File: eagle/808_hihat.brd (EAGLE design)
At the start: 100 x 80 mm, 103 parts, among them IC1 TL072P, IC3 TL071P, Q1 2N3904, Q10 2N3904, Q11 2N3904, Q12 2N3904, Q13 2N3906, Q14 2N3906, Q2 2N3904, Q3 2N3904, Q4 2N3904, Q5 2N3904, Q6 2N3904, Q7 2N3904, Q8 2N3904, Q9 2N3904

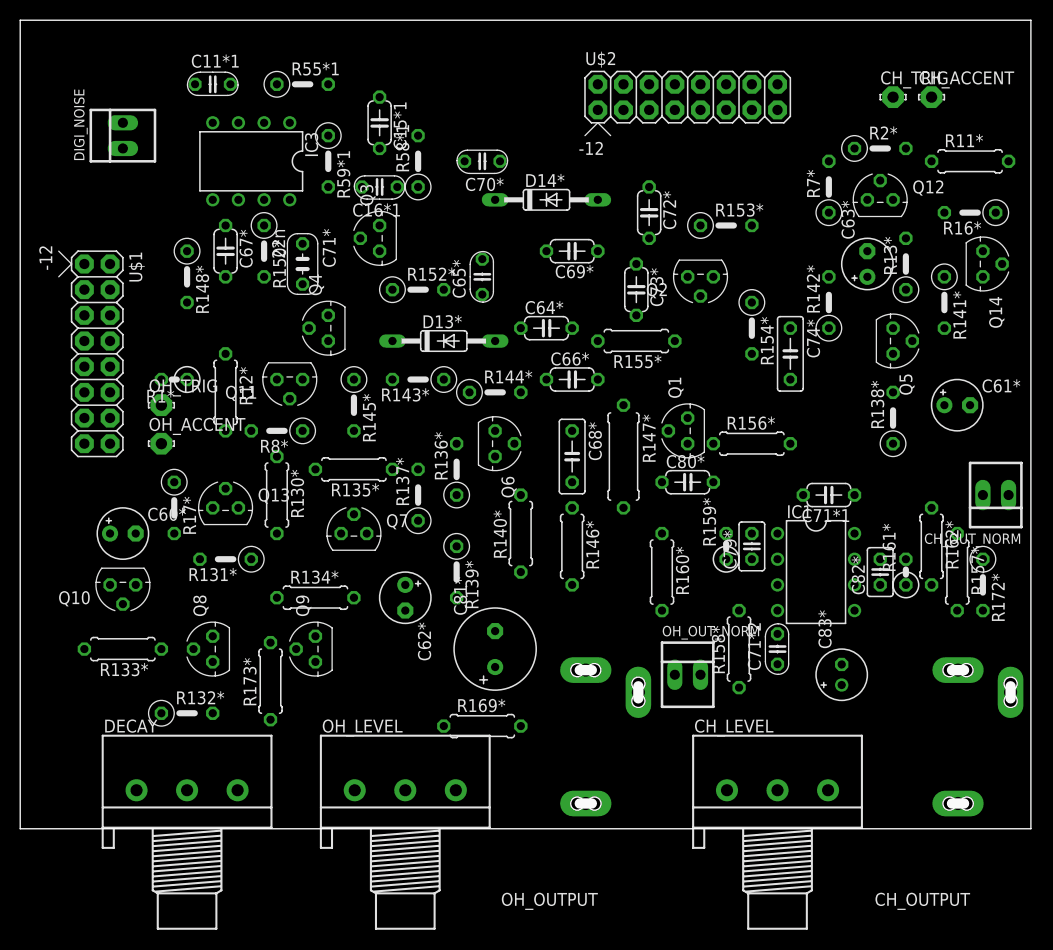
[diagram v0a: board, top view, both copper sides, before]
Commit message: 95pct5 ar
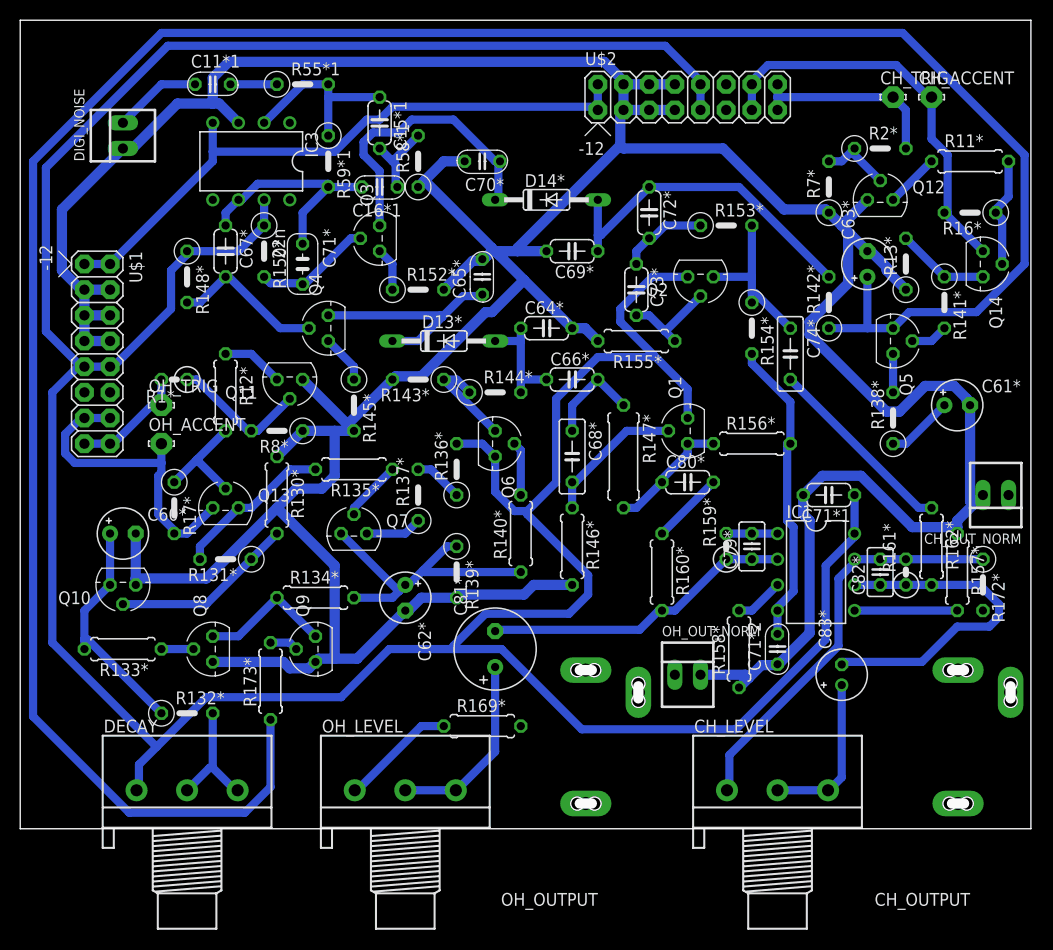
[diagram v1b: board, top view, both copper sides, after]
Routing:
- net GND: track 0.00 -> 422.0 mm
- net +12V: track 0.00 -> 349.2 mm
- net N$581: track 0.00 -> 236.3 mm
- net -12V: track 0.00 -> 93.9 mm
- net N$603: track 0.00 -> 40.8 mm
- net .: track 0.00 -> 40.4 mm
- net N$601: track 0.00 -> 34.0 mm
- net N$220: track 0.00 -> 33.6 mm
- net N$17: track 0.00 -> 31.5 mm
- net N$598: track 0.00 -> 31.0 mm
- net N$573: track 0.00 -> 30.1 mm
- net N$587: track 0.00 -> 29.1 mm
- net N$576: track 0.00 -> 23.1 mm
- net TO_HH: track 0.00 -> 22.9 mm
- net N$588: track 0.00 -> 22.2 mm
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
